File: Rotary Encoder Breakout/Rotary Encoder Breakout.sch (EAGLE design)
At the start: 2 parts, among them P1 HDR-4, SW1 SWITCH-ALPS_EC12E_SW

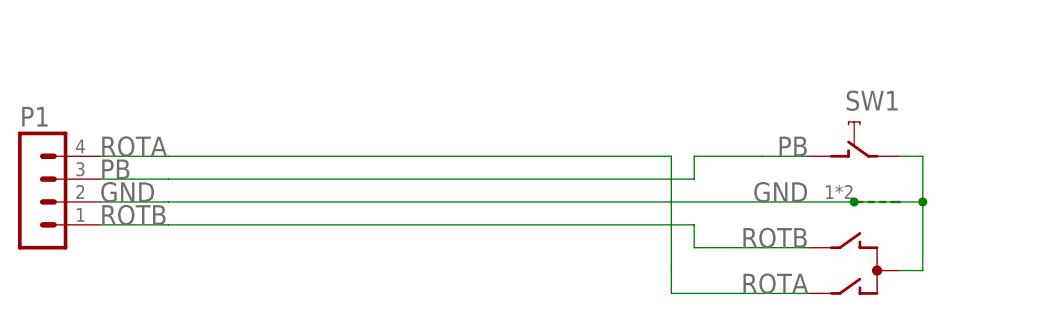
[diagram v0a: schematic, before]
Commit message: Updated part
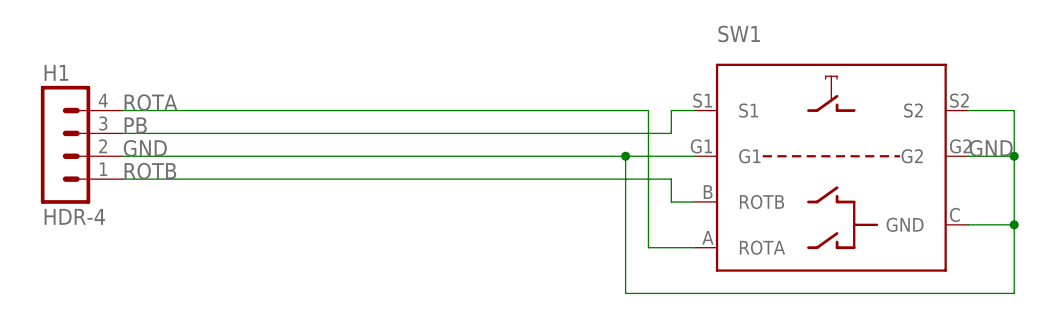
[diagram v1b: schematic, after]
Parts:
- removed P1: HDR-4, Donnie:HDR-4
- added H1: HDR-4, Donnie:HDR-4
- SW1: value SWITCH-ALPS_EC12E_SW -> (none); device Donnie:SWITCH-ALPS_EC12E_SW -> LBussy:ACZ11VERTICAL
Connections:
- net GND: now also H1.2, SW1.G1, SW1.G2, SW1.GND, SW1.S2; no longer P1.2, SW1G$1.C, SW1G$2.E, SW1G$3.1
- net PB: now also H1.3, SW1.S1; no longer P1.3, SW1G$2.D
- net ROTA: now also H1.4, SW1.ROTA; no longer P1.4, SW1G$1.A
- net ROTB: now also H1.1, SW1.ROTB; no longer P1.1, SW1G$1.B
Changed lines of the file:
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@@
 <?xml version="1.0" encoding="utf-8"?>
 <!DOCTYPE eagle SYSTEM "eagle.dtd">
-<eagle version="9.5.2">
+<eagle version="7.7.0">
 <drawing>
 <settings>
@@
 <layer number="91" name="Nets" color="2" fill="1" visible="yes" active="yes"/>
 <layer number="92" name="Busses" color="1" fill="1" visible="yes" active="yes"/>
-<layer number="93" name="Pins" color="2" fill="1" visible="no" active="yes"/>
+<layer number="93" name="Pins" color="2" fill="1" visible="yes" active="yes"/>
 <layer number="94" name="Symbols" color="4" fill="1" visible="yes" active="yes"/>
 <layer number="95" name="Names" color="7" fill="1" visible="yes" active="yes"/>
@@
 </classes>
 <parts>
-<part name="SW1" library="Donnie" deviceset="SWITCH-ALPS_EC12E_SW" device=""/>
-<part name="P1" library="Donnie" deviceset="HDR-4" device=""/>
-<part name="FRAME1" library="frames" library_urn="urn:adsk.eagle:library:229" deviceset="LETTER_L" device=""/>
+<part name="FRAME1" library="frames" deviceset="LETTER_L" device="" value=" "/>
+<part name="SW1" library="LBussy" deviceset="ACZ11" device="VERTICAL" value=" "/>
+<part name="H1" library="Donnie" deviceset="HDR-4" device=""/>
 </parts>
 <sheets>
@@
 </plain>
 <instances>
-<instance part="SW1" gate="G$1" x="167.64" y="86.36" smashed="yes" rot="R90"/>
-<instance part="SW1" gate="G$2" x="165.1" y="99.06" smashed="yes" rot="MR0">
-<attribute name="PART" x="170.18" y="104.14" size="2.1844" layer="95" font="vector" rot="MR0"/>
-</instance>
-<instance part="SW1" gate="G$3" x="165.1" y="93.98" smashed="yes"/>
-<instance part="P1" gate="1" x="73.66" y="91.44" smashed="yes">
-<attribute name="NAME" x="72.39" y="102.362" size="2.1844" layer="95" font="vector"/>
-</instance>
 <instance part="FRAME1" gate="G$1" x="0" y="0" smashed="yes"/>
 <instance part="FRAME1" gate="G$2" x="147.32" y="0" smashed="yes">
@@
 <attribute name="DRAWING_NAME" x="165.1" y="19.05" size="2.54" layer="94"/>
 </instance>
+<instance part="SW1" gate="G$1" x="162.56" y="96.52" smashed="yes">
+<attribute name="NAME" x="149.86" y="111.76" size="1.778" layer="95" font="vector"/>
+<attribute name="VALUE" x="149.86" y="83.82" size="2.1844" layer="96" font="vector" align="top-left"/>
+</instance>
+<instance part="H1" gate="1" x="76.2" y="96.52" smashed="yes">
+<attribute name="VALUE" x="74.93" y="91.44" size="1.778" layer="96" font="vector"/>
+<attribute name="NAME" x="74.93" y="107.442" size="1.778" layer="95" font="vector"/>
+</instance>
 </instances>
 <busses>
@@
 <net name="GND" class="0">
 <segment>
-<pinref part="SW1" gate="G$3" pin="1"/>
-<wire x1="165.1" y1="93.98" x2="154.94" y2="93.98" width="0.1524" layer="91"/>
-<label x="160.02" y="93.98" size="2.1844" layer="95" font="vector" align="bottom-right"/>
-<pinref part="SW1" gate="G$1" pin="C"/>
-<wire x1="172.72" y1="93.98" x2="172.72" y2="86.36" width="0.1524" layer="91"/>
-<wire x1="172.72" y1="86.36" x2="170.18" y2="86.36" width="0.1524" layer="91"/>
-<wire x1="165.1" y1="93.98" x2="172.72" y2="93.98" width="0.1524" layer="91"/>
-<junction x="165.1" y="93.98"/>
-<pinref part="SW1" gate="G$2" pin="E"/>
-<wire x1="170.18" y1="99.06" x2="172.72" y2="99.06" width="0.1524" layer="91"/>
-<wire x1="172.72" y1="99.06" x2="172.72" y2="93.98" width="0.1524" layer="91"/>
-<junction x="172.72" y="93.98"/>
-<pinref part="P1" gate="1" pin="2"/>
-<wire x1="81.28" y1="93.98" x2="88.9" y2="93.98" width="0.1524" layer="91"/>
-<label x="81.28" y="93.98" size="2.1844" layer="95" font="vector"/>
-<wire x1="88.9" y1="93.98" x2="154.94" y2="93.98" width="0.1524" layer="91"/>
+<pinref part="SW1" gate="G$1" pin="G2"/>
+<label x="177.8" y="99.06" size="1.778" layer="95"/>
+<pinref part="SW1" gate="G$1" pin="S2"/>
+<wire x1="177.8" y1="104.14" x2="182.88" y2="104.14" width="0.1524" layer="91"/>
+<wire x1="182.88" y1="104.14" x2="182.88" y2="99.06" width="0.1524" layer="91"/>
+<wire x1="182.88" y1="99.06" x2="177.8" y2="99.06" width="0.1524" layer="91"/>
+<pinref part="SW1" gate="G$1" pin="GND"/>
+<wire x1="182.88" y1="99.06" x2="182.88" y2="91.44" width="0.1524" layer="91"/>
+<wire x1="182.88" y1="91.44" x2="177.8" y2="91.44" width="0.1524" layer="91"/>
+<junction x="182.88" y="99.06"/>
+<wire x1="182.88" y1="91.44" x2="182.88" y2="83.82" width="0.1524" layer="91"/>
+<wire x1="182.88" y1="83.82" x2="139.7" y2="83.82" width="0.1524" layer="91"/>
+<junction x="182.88" y="91.44"/>
+<pinref part="H1" gate="1" pin="2"/>
+<pinref part="SW1" gate="G$1" pin="G1"/>
+<wire x1="83.82" y1="99.06" x2="139.7" y2="99.06" width="0.1524" layer="91"/>
+<label x="83.82" y="99.06" size="1.778" layer="95" font="vector"/>
+<wire x1="139.7" y1="99.06" x2="147.32" y2="99.06" width="0.1524" layer="91"/>
+<wire x1="139.7" y1="83.82" x2="139.7" y2="99.06" width="0.1524" layer="91"/>
+<junction x="139.7" y="99.06"/>
 </segment>
 </net>
 <net name="ROTA" class="0">
 <segment>
-<pinref part="P1" gate="1" pin="4"/>
-<wire x1="81.28" y1="99.06" x2="88.9" y2="99.06" width="0.1524" layer="91"/>
-<label x="81.28" y="99.06" size="2.1844" layer="95" font="vector"/>
-<wire x1="88.9" y1="99.06" x2="144.78" y2="99.06" width="0.1524" layer="91"/>
-<wire x1="144.78" y1="99.06" x2="144.78" y2="86.36" width="0.1524" layer="91"/>
-<pinref part="SW1" gate="G$1" pin="A"/>
-<wire x1="160.02" y1="83.82" x2="154.94" y2="83.82" width="0.1524" layer="91"/>
-<label x="160.02" y="83.82" size="2.1844" layer="95" font="vector" align="bottom-right"/>
-<wire x1="144.78" y1="86.36" x2="144.78" y2="83.82" width="0.1524" layer="91"/>
-<wire x1="144.78" y1="83.82" x2="154.94" y2="83.82" width="0.1524" layer="91"/>
+<pinref part="H1" gate="1" pin="4"/>
+<wire x1="83.82" y1="104.14" x2="142.24" y2="104.14" width="0.1524" layer="91"/>
+<wire x1="142.24" y1="104.14" x2="142.24" y2="88.9" width="0.1524" layer="91"/>
+<pinref part="SW1" gate="G$1" pin="ROTA"/>
+<wire x1="142.24" y1="88.9" x2="147.32" y2="88.9" width="0.1524" layer="91"/>
+<label x="83.82" y="104.14" size="1.778" layer="95" font="vector"/>
 </segment>
 </net>
 <net name="PB" class="0">
 <segment>
-<pinref part="P1" gate="1" pin="3"/>
-<wire x1="81.28" y1="96.52" x2="88.9" y2="96.52" width="0.1524" layer="91"/>
-<label x="81.28" y="96.52" size="2.1844" layer="95" font="vector"/>
-<wire x1="88.9" y1="96.52" x2="147.32" y2="96.52" width="0.1524" layer="91"/>
-<wire x1="147.32" y1="96.52" x2="147.32" y2="99.06" width="0.1524" layer="91"/>
-<pinref part="SW1" gate="G$2" pin="D"/>
-<wire x1="160.02" y1="99.06" x2="154.94" y2="99.06" width="0.1524" layer="91"/>
-<label x="160.02" y="99.06" size="2.1844" layer="95" align="bottom-right"/>
-<wire x1="147.32" y1="99.06" x2="154.94" y2="99.06" width="0.1524" layer="91"/>
+<pinref part="SW1" gate="G$1" pin="S1"/>
+<wire x1="147.32" y1="104.14" x2="144.78" y2="104.14" width="0.1524" layer="91"/>
+<wire x1="144.78" y1="104.14" x2="144.78" y2="101.6" width="0.1524" layer="91"/>
+<pinref part="H1" gate="1" pin="3"/>
+<wire x1="144.78" y1="101.6" x2="83.82" y2="101.6" width="0.1524" layer="91"/>
+<label x="83.82" y="101.6" size="1.778" layer="95" font="vector"/>
 </segment>
 </net>
 <net name="ROTB" class="0">
 <segment>
-<pinref part="P1" gate="1" pin="1"/>
-<wire x1="81.28" y1="91.44" x2="88.9" y2="91.44" width="0.1524" layer="91"/>
-<label x="81.28" y="91.44" size="2.1844" layer="95" font="vector"/>
-<wire x1="88.9" y1="91.44" x2="147.32" y2="91.44" width="0.1524" layer="91"/>
-<wire x1="147.32" y1="91.44" x2="147.32" y2="88.9" width="0.1524" layer="91"/>
-<pinref part="SW1" gate="G$1" pin="B"/>
-<wire x1="160.02" y1="88.9" x2="154.94" y2="88.9" width="0.1524" layer="91"/>
-<label x="160.02" y="88.9" size="2.1844" layer="95" font="vector" align="bottom-right"/>
-<wire x1="147.32" y1="88.9" x2="154.94" y2="88.9" width="0.1524" layer="91"/>
+<pinref part="H1" gate="1" pin="1"/>
+<wire x1="83.82" y1="96.52" x2="144.78" y2="96.52" width="0.1524" layer="91"/>
+<wire x1="144.78" y1="96.52" x2="144.78" y2="93.98" width="0.1524" layer="91"/>
+<pinref part="SW1" gate="G$1" pin="ROTB"/>
+<wire x1="144.78" y1="93.98" x2="147.32" y2="93.98" width="0.1524" layer="91"/>
+<label x="83.82" y="96.52" size="1.778" layer="95" font="vector"/>
 </segment>
 </net>
@@
 </sheet>
 </sheets>
-<errors>
-</errors>
 </schematic>
 </drawing>
-<compatibility>
-<note version="8.2" severity="warning">
-Since Version 8.2, EAGLE supports online libraries. The ids
-of those online libraries will not be understood (or retained)
-with this version.
-</note>
-<note version="8.3" severity="warning">
-Since Version 8.3, EAGLE supports URNs for individual library
-assets (packages, symbols, and devices). The URNs of those assets
-will not be understood (or retained) with this version.
-</note>
-<note version="9.0" severity="warning">
-Since Version 9.0, EAGLE supports the align property for labels.
-Labels in schematic will not be understood with this version. Update EAGLE to the latest version
-for full support of labels.
-</note>
-</compatibility>
 </eagle>
